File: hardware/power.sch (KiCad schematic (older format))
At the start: 40 parts, among them U200 SY8089AAC, U220 PAM2305CGFADJ, U230 PAM2305CGFADJ, U250 PAM2305CGFADJ, U260 NCP707_XDFN4

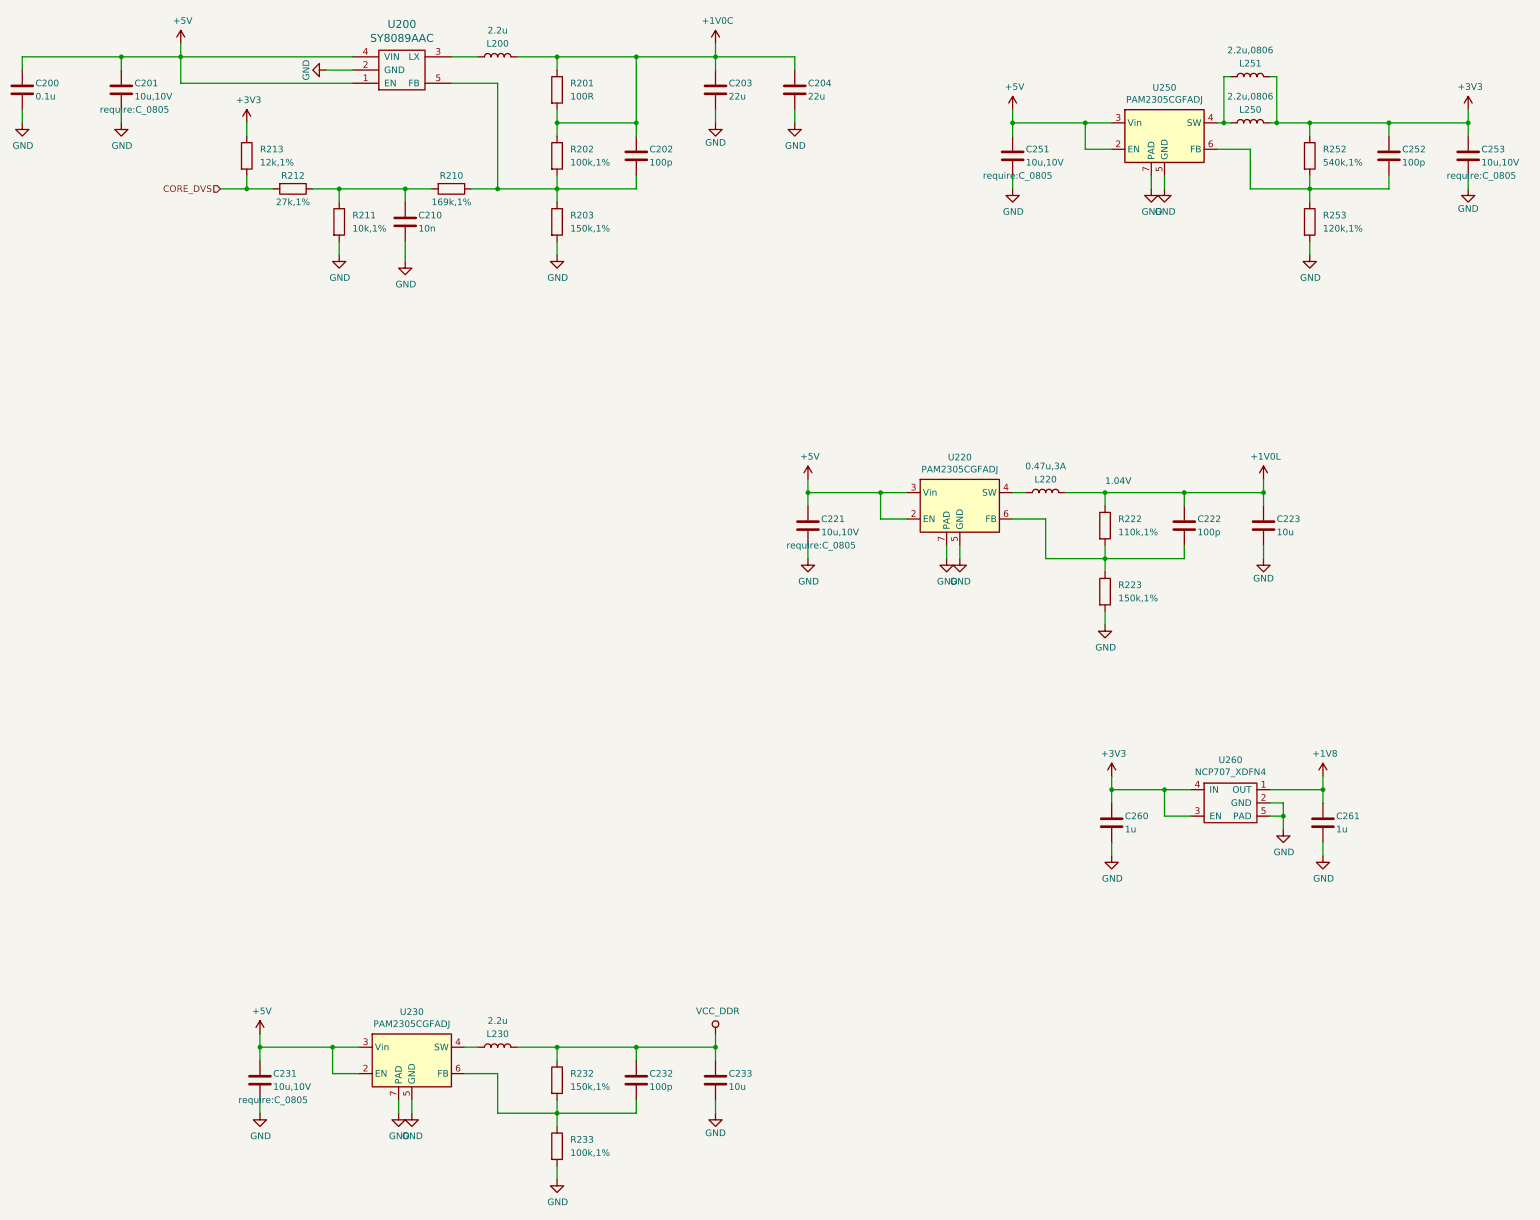
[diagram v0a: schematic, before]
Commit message: wip
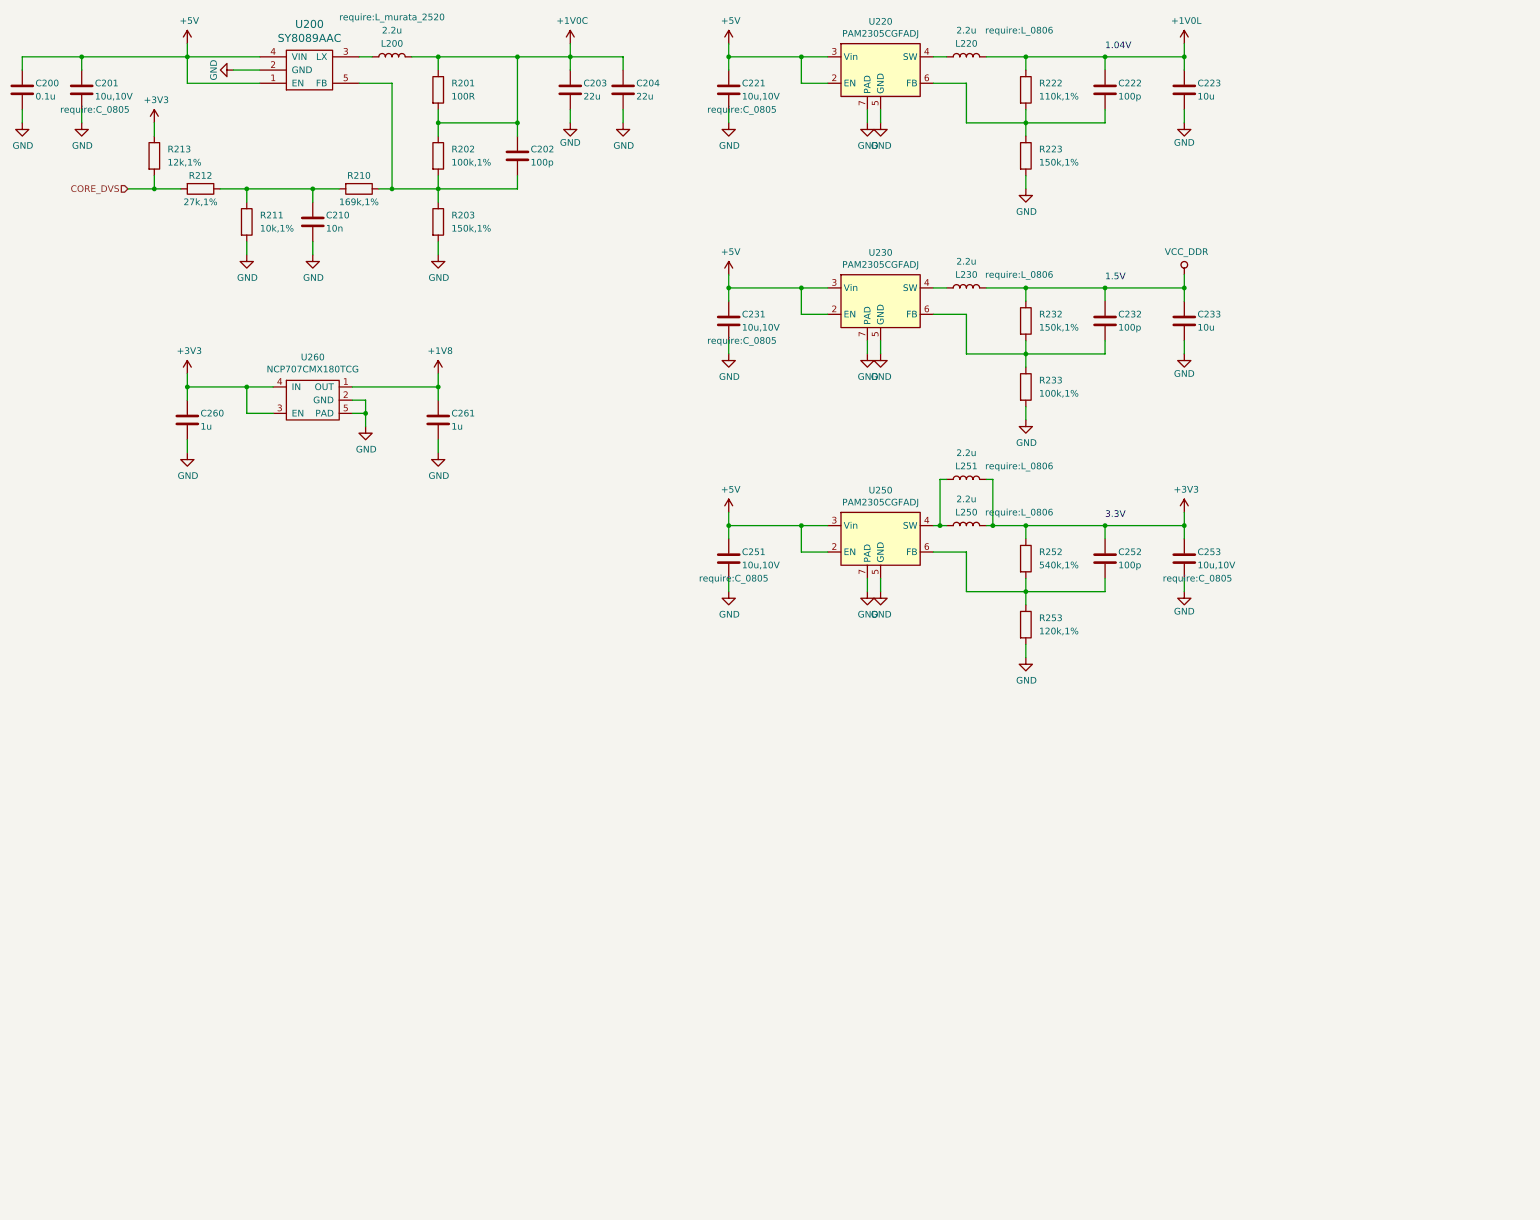
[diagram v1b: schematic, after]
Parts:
- L220: value 0.47u,3A -> 2.2u
- L250, L251: value 2.2u,0806 -> 2.2u
- U260: value NCP707_XDFN4 -> NCP707CMX180TCG
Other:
- note added: "1.5V"
- note added: "3.3V"
- moved on the sheet: C201, C202, C203, C204, C210, C221, C222, C223, C231, C232, C233, C251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
